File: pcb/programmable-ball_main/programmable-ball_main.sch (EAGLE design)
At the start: 2 parts, among them J1 USB4125-GF-A_REVA2, U1 MDBT50Q-1MV2

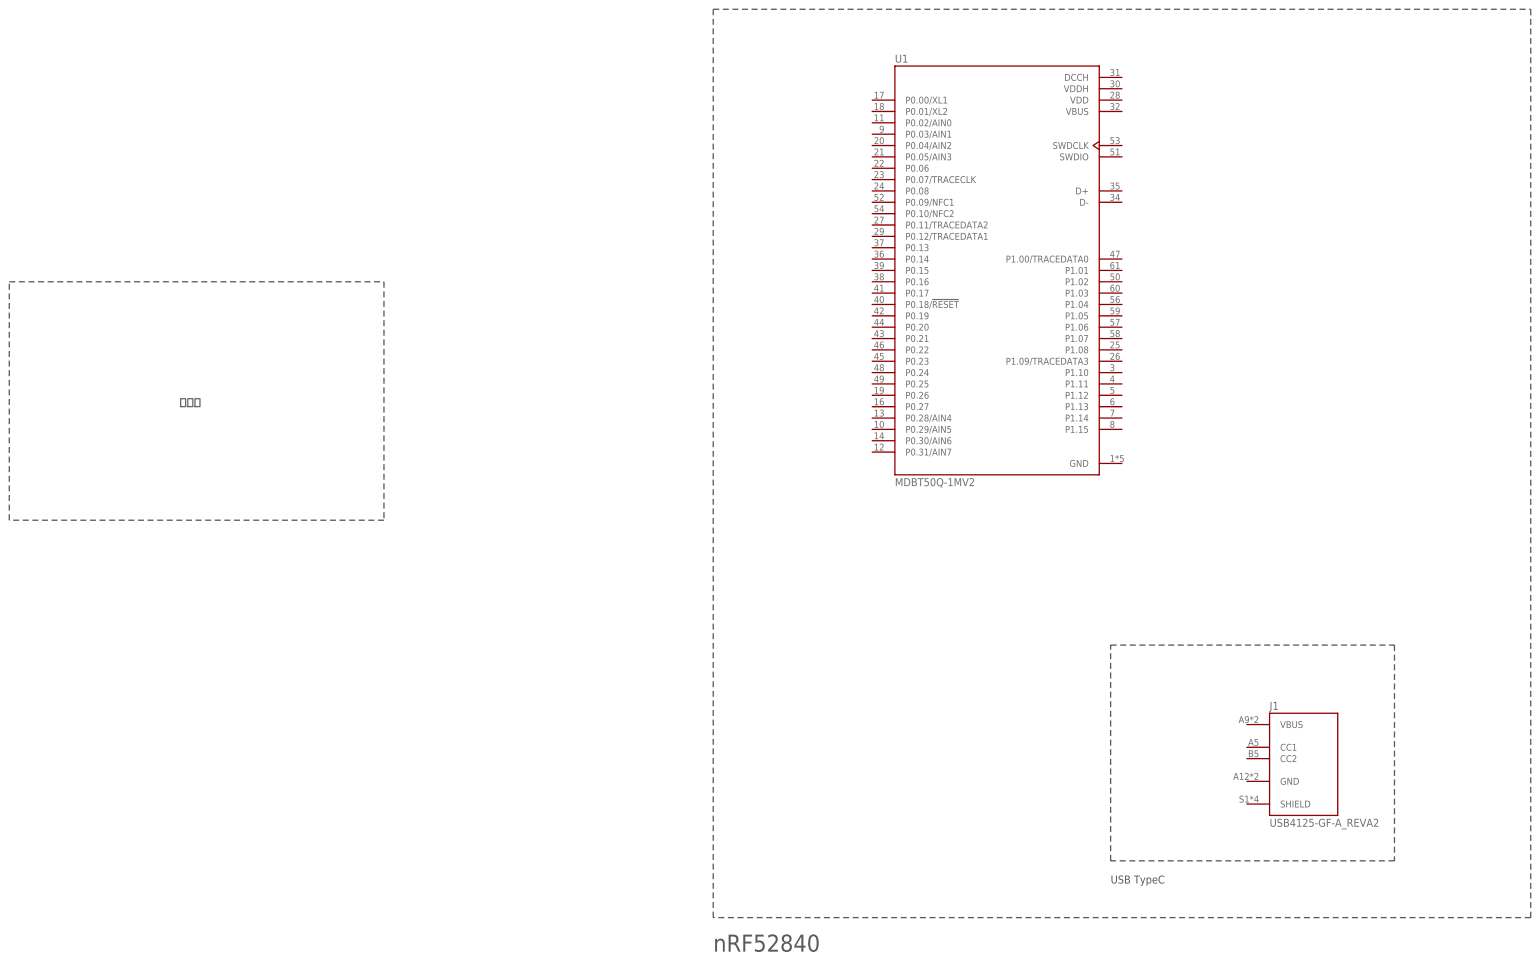
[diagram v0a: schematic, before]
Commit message: 軽微な修正
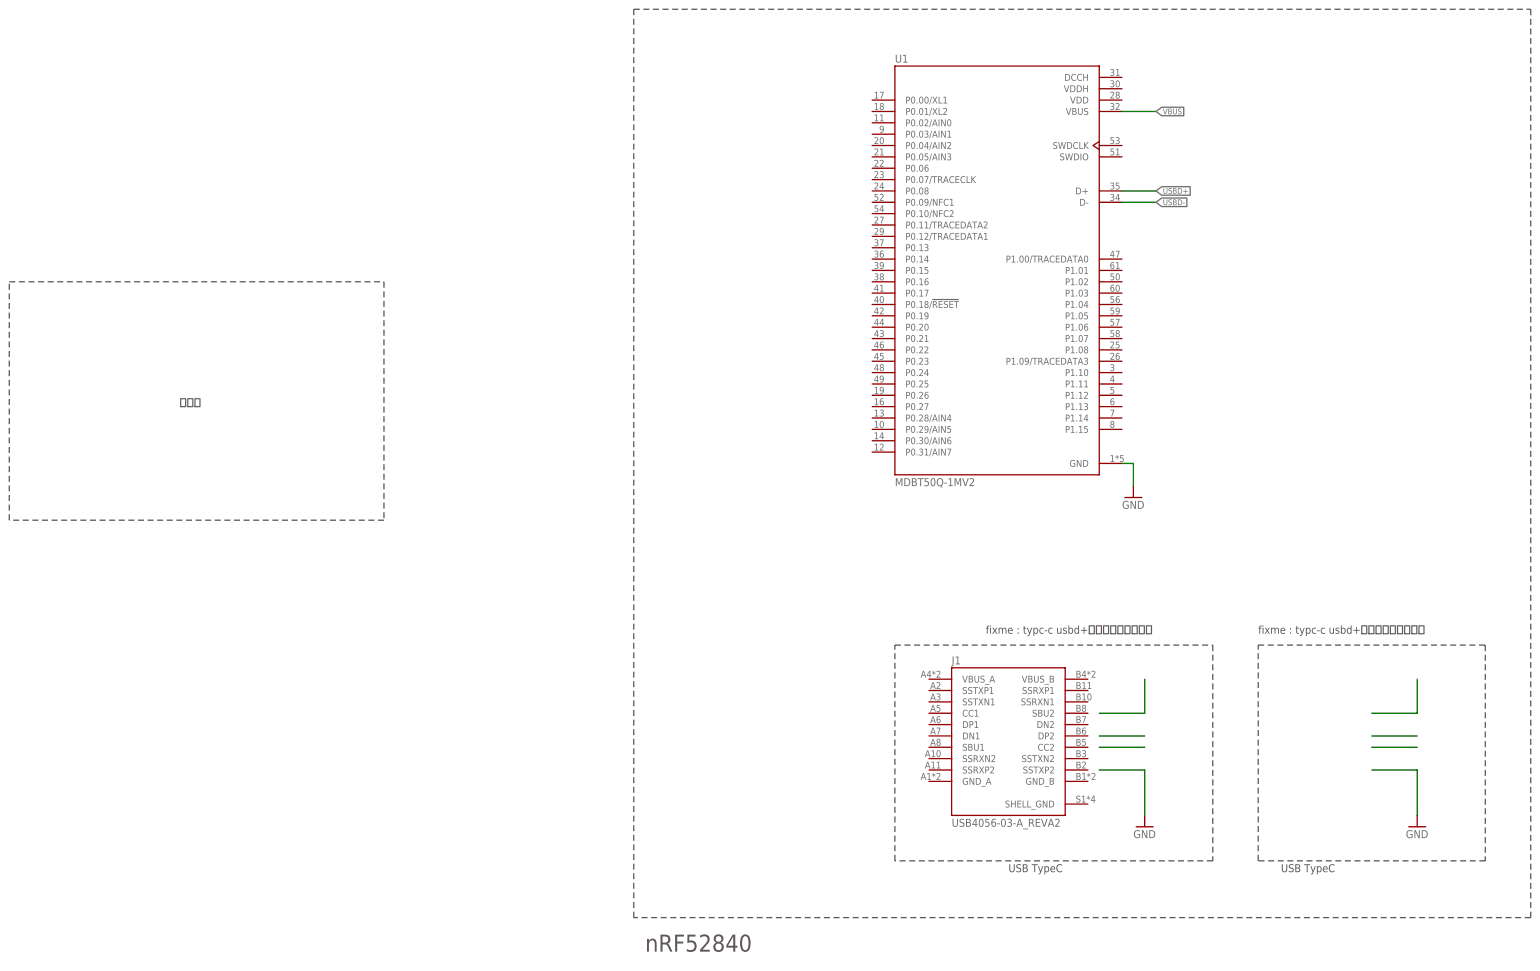
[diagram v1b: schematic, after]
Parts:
- J1: value USB4125-GF-A_REVA2 -> USB4056-03-A_REVA2; device USB4125-GF-A_REVA2:USB4125-GF-A_REVA2 -> USB4056-03-A_REVA2:USB4056-03-A_REVA2
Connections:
- new net GND: U1.GND
- new net USBD+: U1.D+
- new net USBD-: U1.D-
- new net VBUS: U1.VBUS
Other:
- note added: "fixme : typc-c usbd+も出せるようにして"
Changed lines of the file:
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@@
 <layers>
 <layer number="1" name="Top" color="4" fill="1" visible="no" active="no"/>
+<layer number="2" name="Route2" color="1" fill="3" visible="no" active="no"/>
+<layer number="3" name="Route3" color="4" fill="3" visible="no" active="no"/>
+<layer number="4" name="Route4" color="1" fill="4" visible="no" active="no"/>
+<layer number="5" name="Route5" color="4" fill="4" visible="no" active="no"/>
+<layer number="6" name="Route6" color="1" fill="8" visible="no" active="no"/>
+<layer number="7" name="Route7" color="4" fill="8" visible="no" active="no"/>
+<layer number="8" name="Route8" color="1" fill="2" visible="no" active="no"/>
+<layer number="9" name="Route9" color="4" fill="2" visible="no" active="no"/>
+<layer number="10" name="Route10" color="1" fill="7" visible="no" active="no"/>
+<layer number="11" name="Route11" color="4" fill="7" visible="no" active="no"/>
+<layer number="12" name="Route12" color="1" fill="5" visible="no" active="no"/>
+<layer number="13" name="Route13" color="4" fill="5" visible="no" active="no"/>
+<layer number="14" name="Route14" color="1" fill="6" visible="no" active="no"/>
+<layer number="15" name="Route15" color="4" fill="6" visible="no" active="no"/>
 <layer number="16" name="Bottom" color="1" fill="1" visible="no" active="no"/>
 <layer number="17" name="Pads" color="2" fill="1" visible="no" active="no"/>
@@
 <part name="FRAME1" library="SparkFun-Retired" deviceset="FRAME-A3" device=""/>
 <part name="U1" library="MDBT50Q-1MV2" deviceset="MDBT50Q-1MV2" device=""/>
-<part name="J1" library="USB4125-GF-A_REVA2" deviceset="USB4125-GF-A_REVA2" device=""/>
+<part name="GND1" library="supply1" library_urn="urn:adsk.eagle:library:371" deviceset="GND" device=""/>
+<part name="GND2" library="supply1" library_urn="urn:adsk.eagle:library:371" deviceset="GND" device=""/>
+<part name="GND3" library="supply1" library_urn="urn:adsk.eagle:library:371" deviceset="GND" device=""/>
+<part name="J1" library="USB4056-03-A_REVA2" deviceset="USB4056-03-A_REVA2" device=""/>
 </parts>
 <sheets>
 <sheet>
 <plain>
-<wire x1="365.76" y1="43.18" x2="182.88" y2="43.18" width="0.1524" layer="97" style="shortdash"/>
-<wire x1="182.88" y1="43.18" x2="182.88" y2="246.38" width="0.1524" layer="97" style="shortdash"/>
-<wire x1="182.88" y1="246.38" x2="365.76" y2="246.38" width="0.1524" layer="97" style="shortdash"/>
+<wire x1="365.76" y1="43.18" x2="165.1" y2="43.18" width="0.1524" layer="97" style="shortdash"/>
+<wire x1="165.1" y1="43.18" x2="165.1" y2="246.38" width="0.1524" layer="97" style="shortdash"/>
+<wire x1="165.1" y1="246.38" x2="365.76" y2="246.38" width="0.1524" layer="97" style="shortdash"/>
 <wire x1="365.76" y1="246.38" x2="365.76" y2="43.18" width="0.1524" layer="97" style="shortdash"/>
-<text x="182.88" y="35.56" size="3.81" layer="97">nRF52840</text>
+<text x="167.64" y="35.56" size="3.81" layer="97">nRF52840</text>
 <wire x1="25.4" y1="185.42" x2="109.22" y2="185.42" width="0.1524" layer="97" style="shortdash"/>
 <wire x1="109.22" y1="185.42" x2="109.22" y2="132.08" width="0.1524" layer="97" style="shortdash"/>
@@
 <wire x1="25.4" y1="132.08" x2="25.4" y2="185.42" width="0.1524" layer="97" style="shortdash"/>
 <text x="63.5" y="157.48" size="1.778" layer="97">電源系</text>
-<wire x1="271.78" y1="104.14" x2="335.28" y2="104.14" width="0.1524" layer="97" style="shortdash"/>
-<wire x1="335.28" y1="104.14" x2="335.28" y2="55.88" width="0.1524" layer="97" style="shortdash"/>
-<wire x1="335.28" y1="55.88" x2="271.78" y2="55.88" width="0.1524" layer="97" style="shortdash"/>
-<wire x1="271.78" y1="55.88" x2="271.78" y2="104.14" width="0.1524" layer="97" style="shortdash"/>
-<text x="271.78" y="50.8" size="1.778" layer="97">USB TypeC</text>
+<wire x1="304.8" y1="104.14" x2="355.6" y2="104.14" width="0.1524" layer="97" style="shortdash"/>
+<wire x1="355.6" y1="104.14" x2="355.6" y2="55.88" width="0.1524" layer="97" style="shortdash"/>
+<wire x1="355.6" y1="55.88" x2="304.8" y2="55.88" width="0.1524" layer="97" style="shortdash"/>
+<wire x1="304.8" y1="55.88" x2="304.8" y2="104.14" width="0.1524" layer="97" style="shortdash"/>
+<text x="309.88" y="53.34" size="1.778" layer="97">USB TypeC</text>
+<text x="304.8" y="106.68" size="1.778" layer="97">fixme : typc-c usbd+も出せるようにして</text>
+<wire x1="223.52" y1="104.14" x2="294.64" y2="104.14" width="0.1524" layer="97" style="shortdash"/>
+<wire x1="294.64" y1="104.14" x2="294.64" y2="55.88" width="0.1524" layer="97" style="shortdash"/>
+<wire x1="294.64" y1="55.88" x2="223.52" y2="55.88" width="0.1524" layer="97" style="shortdash"/>
+<wire x1="223.52" y1="55.88" x2="223.52" y2="104.14" width="0.1524" layer="97" style="shortdash"/>
+<text x="248.92" y="53.34" size="1.778" layer="97">USB TypeC</text>
+<text x="243.84" y="106.68" size="1.778" layer="97">fixme : typc-c usbd+も出せるようにして</text>
 </plain>
 <instances>
@@
 <attribute name="VALUE" x="223.52" y="139.7" size="1.778" layer="96"/>
 </instance>
-<instance part="J1" gate="G$1" x="314.96" y="78.74" smashed="yes">
-<attribute name="NAME" x="307.34" y="89.662" size="1.778" layer="95"/>
-<attribute name="VALUE" x="307.34" y="65.278" size="1.778" layer="96" rot="MR180"/>
+<instance part="GND1" gate="1" x="276.86" y="137.16" smashed="yes">
+<attribute name="VALUE" x="274.32" y="134.62" size="1.778" layer="96"/>
+</instance>
+<instance part="GND2" gate="1" x="340.36" y="63.5" smashed="yes">
+<attribute name="VALUE" x="337.82" y="60.96" size="1.778" layer="96"/>
+</instance>
+<instance part="GND3" gate="1" x="279.4" y="63.5" smashed="yes">
+<attribute name="VALUE" x="276.86" y="60.96" size="1.778" layer="96"/>
+</instance>
+<instance part="J1" gate="G$1" x="248.92" y="83.82" smashed="yes">
+<attribute name="NAME" x="236.22" y="99.822" size="1.778" layer="95"/>
+<attribute name="VALUE" x="236.22" y="65.278" size="1.778" layer="96" rot="MR180"/>
 </instance>
 </instances>
@@
 </busses>
 <nets>
+<net name="GND" class="0">
+<segment>
+<pinref part="U1" gate="G$1" pin="GND"/>
+<pinref part="GND1" gate="1" pin="GND"/>
+<wire x1="274.32" y1="144.78" x2="276.86" y2="144.78" width="0.1524" layer="91"/>
+<wire x1="276.86" y1="144.78" x2="276.86" y2="139.7" width="0.1524" layer="91"/>
+</segment>
+<segment>
+<pinref part="GND2" gate="1" pin="GND"/>
+<wire x1="330.2" y1="76.2" x2="340.36" y2="76.2" width="0.1524" layer="91"/>
+<wire x1="340.36" y1="76.2" x2="340.36" y2="66.04" width="0.1524" layer="91"/>
+</segment>
+<segment>
+<pinref part="GND3" gate="1" pin="GND"/>
+<wire x1="269.24" y1="76.2" x2="279.4" y2="76.2" width="0.1524" layer="91"/>
+<wire x1="279.4" y1="76.2" x2="279.4" y2="66.04" width="0.1524" layer="91"/>
+</segment>
+</net>
+<net name="VBUS" class="0">
+<segment>
+<pinref part="U1" gate="G$1" pin="VBUS"/>
+<wire x1="274.32" y1="223.52" x2="281.94" y2="223.52" width="0.1524" layer="91"/>
+<label x="281.94" y="223.52" size="1.27" layer="95" xref="yes"/>
+</segment>
+</net>
+<net name="USBD+" class="0">
+<segment>
+<pinref part="U1" gate="G$1" pin="D+"/>
+<wire x1="274.32" y1="205.74" x2="281.94" y2="205.74" width="0.1524" layer="91"/>
+<label x="281.94" y="205.74" size="1.27" layer="95" xref="yes"/>
+</segment>
+</net>
+<net name="USBD-" class="0">
+<segment>
+<pinref part="U1" gate="G$1" pin="D-"/>
+<wire x1="274.32" y1="203.2" x2="281.94" y2="203.2" width="0.1524" layer="91"/>
+<label x="281.94" y="203.2" size="1.27" layer="95" xref="yes"/>
+</segment>
+</net>
+<net name="N$1" class="0">
+<segment>
+<wire x1="330.2" y1="88.9" x2="340.36" y2="88.9" width="0.1524" layer="91"/>
+<wire x1="340.36" y1="88.9" x2="340.36" y2="96.52" width="0.1524" layer="91"/>
+</segment>
+</net>
+<net name="N$2" class="0">
+<segment>
+<wire x1="330.2" y1="83.82" x2="340.36" y2="83.82" width="0.1524" layer="91"/>
+</segment>
+</net>
+<net name="N$3" class="0">
+<segment>
+<wire x1="330.2" y1="81.28" x2="340.36" y2="81.28" width="0.1524" layer="91"/>
+</segment>
+</net>
+<net name="N$4" class="0">
+<segment>
+<wire x1="269.24" y1="88.9" x2="279.4" y2="88.9" width="0.1524" layer="91"/>
+<wire x1="279.4" y1="88.9" x2="279.4" y2="96.52" width="0.1524" layer="91"/>
+</segment>
+</net>
+<net name="N$5" class="0">
+<segment>
+<wire x1="269.24" y1="83.82" x2="279.4" y2="83.82" width="0.1524" layer="91"/>
+</segment>
+</net>
+<net name="N$6" class="0">
+<segment>
+<wire x1="269.24" y1="81.28" x2="279.4" y2="81.28" width="0.1524" layer="91"/>
+</segment>
+</net>
 </nets>
 </sheet>
@@
 </schematic>
 </drawing>
+<compatibility>
+<note version="8.2" severity="warning">
+Since Version 8.2, EAGLE supports online libraries. The ids
+of those online libraries will not be understood (or retained)
+with this version.
+</note>
+<note version="8.3" severity="warning">
+Since Version 8.3, EAGLE supports URNs for individual library
+assets (packages, symbols, and devices). The URNs of those assets
+will not be understood (or retained) with this version.
+</note>
+</compatibility>
 </eagle>

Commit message: usb typeC周り実装 #4
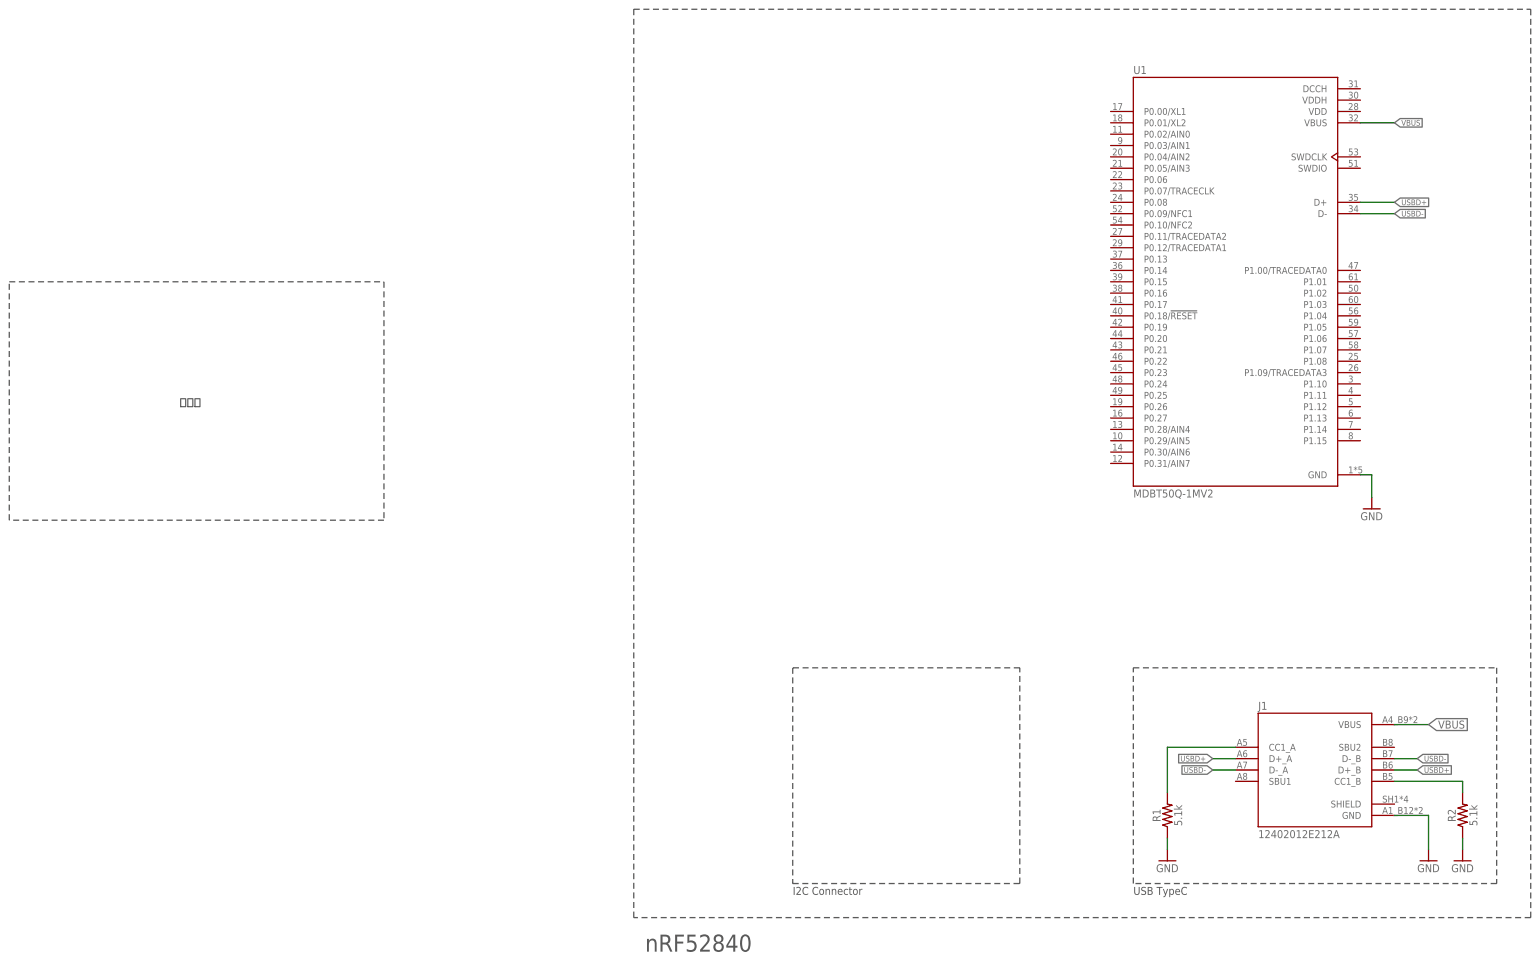
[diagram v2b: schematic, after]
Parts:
- added R1, R2: 5.1k, SparkFun-Resistors:5.1KOHM-0402T-1/16W-1%
- J1: value USB4056-03-A_REVA2 -> 12402012E212A; device USB4056-03-A_REVA2:USB4056-03-A_REVA2 -> 12402012E212A:12402012E212A
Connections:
- new net N$1: J1.CC1_A, R1.2
- new net N$2: J1.CC1_B, R2.2
- net GND: now also J1.GND, R1.1, R2.1
- net USBD+: now also J1.D+_A, J1.D+_B
- net USBD-: now also J1.D-_A, J1.D-_B
- net VBUS: now also J1.VBUS
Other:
- note added: "I2C Connector"
- note removed: "fixme : typc-c usbd+も出せるようにして"
- moved on the sheet: U1
